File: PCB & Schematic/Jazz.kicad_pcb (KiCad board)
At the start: 4 copper layers, 38.5 x 30.2 mm, 29 parts, among them P1 MountingHole_Pad, U1 XIAO-nRF52840-DIP, U2 TLV75533PDBVR, U3 BQ24040DSQT, U4 MAX98357AETE+T

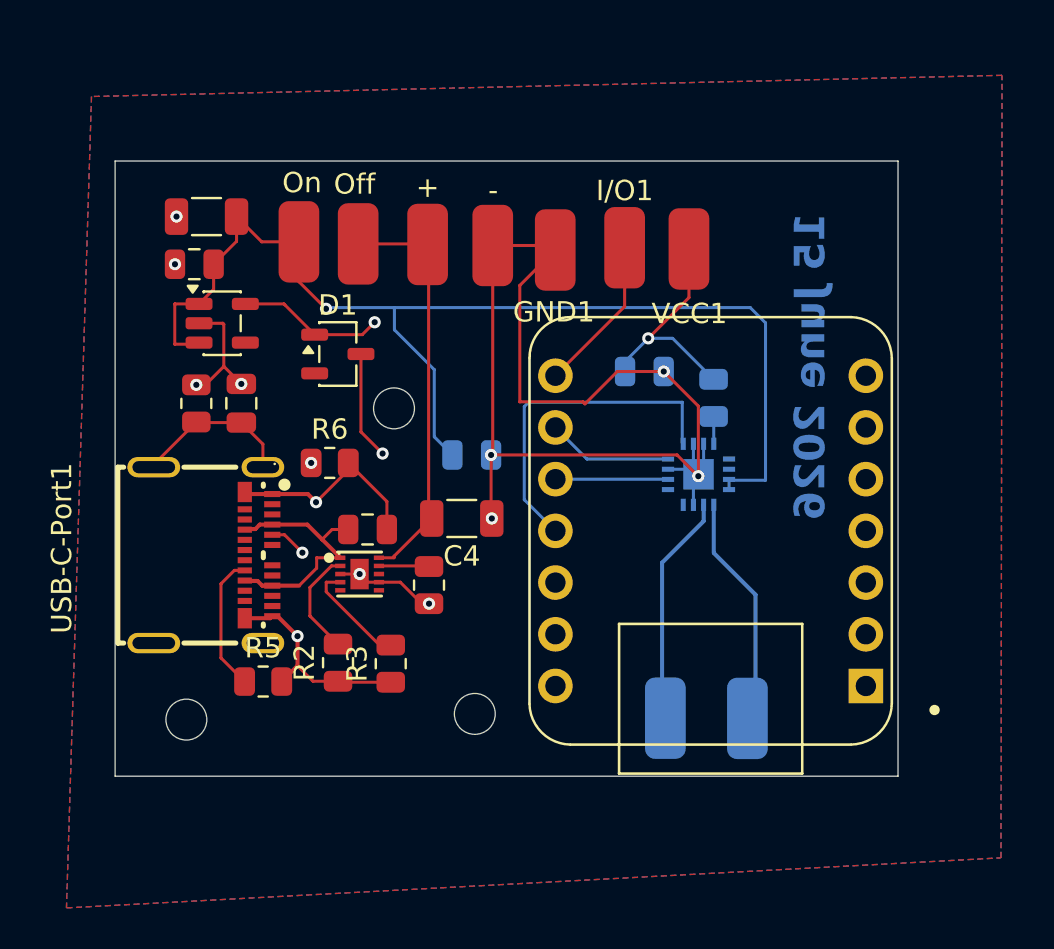
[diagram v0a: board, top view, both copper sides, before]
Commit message: Possibly Done
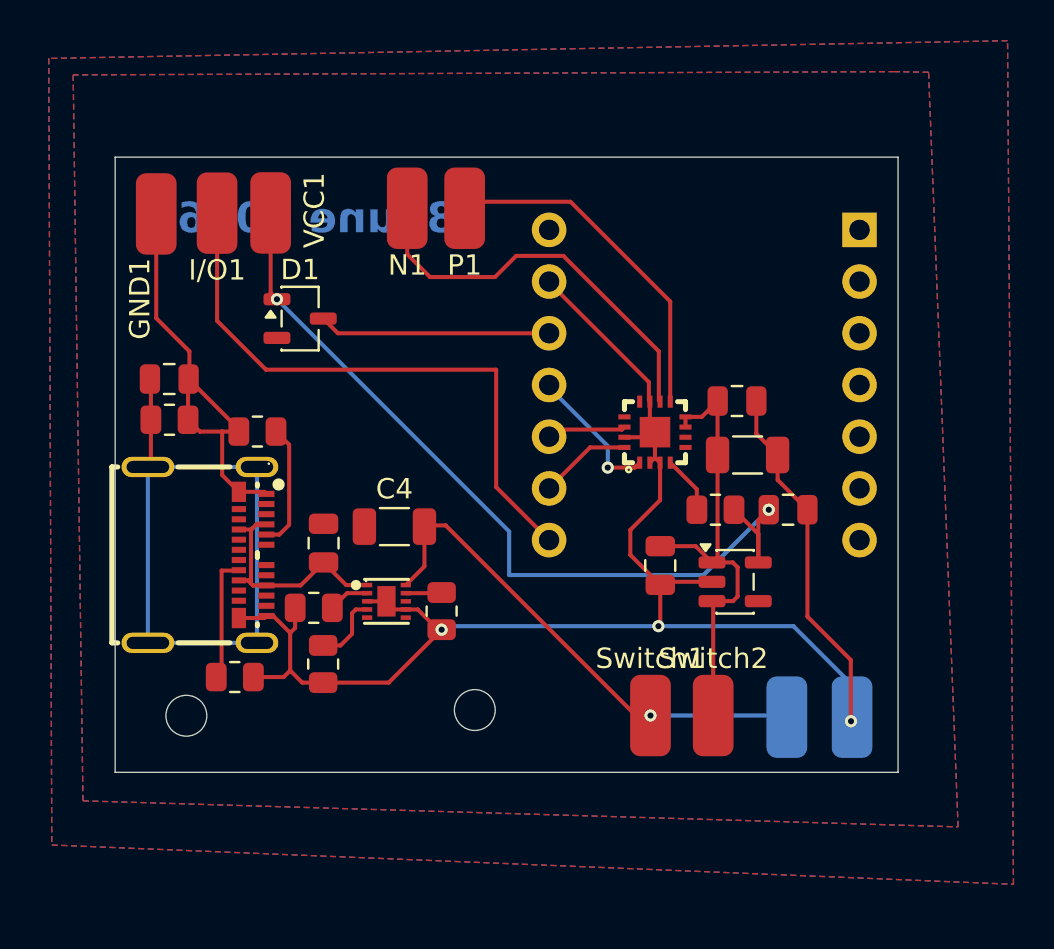
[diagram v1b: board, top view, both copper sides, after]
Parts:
- removed +, -, Off, On: MountingHole_Pad, Connector_Wire:SolderWirePad_1x01_SMD_2x4mm
- removed U1: XIAO-nRF52840-DIP, Seeed Studio XIAO Series Library:XIAO-Generic-Thruhole-14P-2.54-21X17.8MM
- added B+1: MountingHole_Pad, Connector_Wire:SolderWirePad_1x01_SMD_2x4mm, B.Cu at (89.1, 79.8)
- added B-1: MountingHole_Pad, Connector_Wire:SolderWirePad_1x01_SMD_2x4mm, B.Cu at (92.3, 79.8)
- added Switch1: MountingHole_Pad, Connector_Wire:SolderWirePad_1x01_SMD_2x4mm, F.Cu at (82.4, 79.7)
- added Switch2: MountingHole_Pad, Connector_Wire:SolderWirePad_1x01_SMD_2x4mm, F.Cu at (85.5, 79.7)
- added U5: XIAO-ESP32-S3-DIP, Seeed Studio XIAO Series Library:XIAO-Generic-Thruhole-14P-2.54-21X17.8MM, B.Cu at (85.0, 63.5)
- C1, C6, N1, P1, R1, U4: moved to F.Cu
- moved C2 29.0 mm to (87.1, 66.9), turned to 0 degrees
- moved P1 28.7 mm to (73.2, 54.8)
- moved U2 28.2 mm to (86.5, 73.1)
- moved N1 28.1 mm to (70.4, 54.8)
- moved C5 27.3 mm to (82.8, 72.3), turned to 90 degrees
- moved VCC1 20.6 mm to (63.7, 55.0)
- moved I/O1 20.1 mm to (61.1, 55.0), turned to 180 degrees
- moved GND1 19.7 mm to (58.1, 55.1)
- moved C1 13.3 mm to (86.6, 64.3)
- moved C6 9.80 mm to (89.1, 69.6)
- moved R1 5.49 mm to (85.6, 69.6), turned to 180 degrees
- moved R6 3.87 mm to (63.1, 65.8), turned to 180 degrees
- moved C7 3.73 mm to (58.7, 63.2), turned to 180 degrees
- moved C4 3.33 mm to (69.8, 70.4), turned to 0 degrees
- moved R3 3.32 mm to (66.3, 77.2)
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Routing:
- net GND: track 150.5 -> 108.6 mm, vias 12 -> 3
- net Switch_OUT: track 57.2 -> 23.1 mm, vias 1 -> 0
- net Pairing-Mode: track 7.70 -> 29.4 mm
- net 3.3V: track 32.4 -> 42.6 mm
- net DIN: track 16.6 -> 6.92 mm, vias 0 -> 1
- net Diode Out: track 20.5 -> 11.4 mm, vias 1 -> 0
- net OUT-N: track 11.4 -> 20.0 mm
- net OUT-P: track 11.5 -> 17.2 mm
- net GROUND: track 27.3 -> 32.5 mm
- net Battery-Rail Out: track 20.6 -> 25.0 mm, vias 0 -> 1
- net Net-(U3-ISET): track 5.28 -> 2.01 mm
- net Net-(U3-PRETERM): track 5.42 -> 3.49 mm
- net LRCK: track 5.54 -> 3.90 mm
- net BCLK: track 6.17 -> 4.53 mm
- net Net-(U4-~{SD_MODE}): track 1.34 -> 2.85 mm
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- added copper zone on B.Cu, net GND
- added copper zone on F.Cu, net GND
- added copper zone on B.Cu, net GROUND
- added copper zone on F.Cu, net GROUND
- removed copper zone on B.Cu, net (none)
- removed copper zone on F.Cu, net (none)
- removed copper zone on In1.Cu, net (none)
- removed copper zone on In2.Cu, net (none)
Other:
- outline, holes or cut-outs redrawn
- copper layers 4 -> 2
- board text added: "28 June 2026"
- board text removed: "15 June 2026"
